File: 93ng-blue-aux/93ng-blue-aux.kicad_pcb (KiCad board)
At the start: 2 copper layers, 100 x 100 mm, 32 parts, among them J1 12V INPUT, J2 ESP32 UART, J3 ESP32 JTAG, J4 AUX OUT, J5 MIC IN, J6 BM62 UART, J7 I-BUS, SW1 SYS CONFIG, U1 ESP32-WROOM-32D, U2 BA33DD0T, U3 MC33897, U4 BM62SPKS1MC2-0001AA

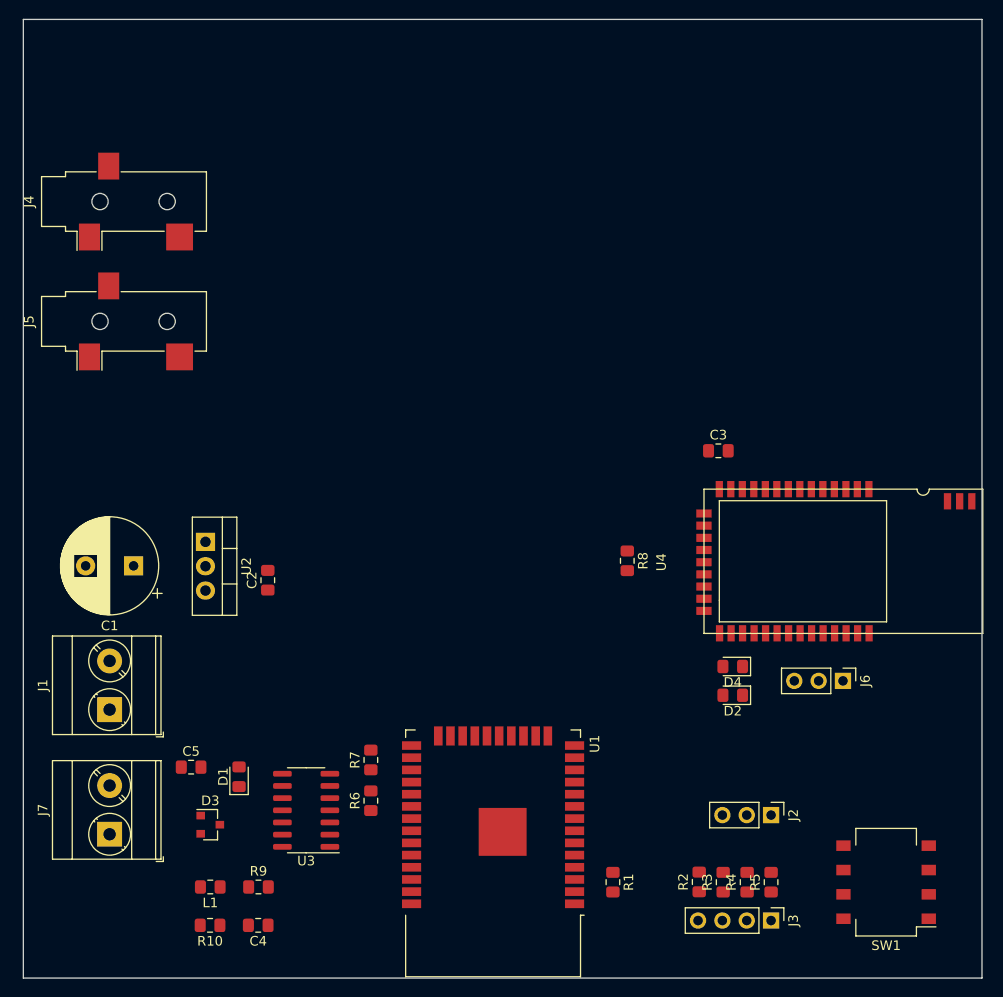
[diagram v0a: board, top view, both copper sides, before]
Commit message: PCB Layout progress.
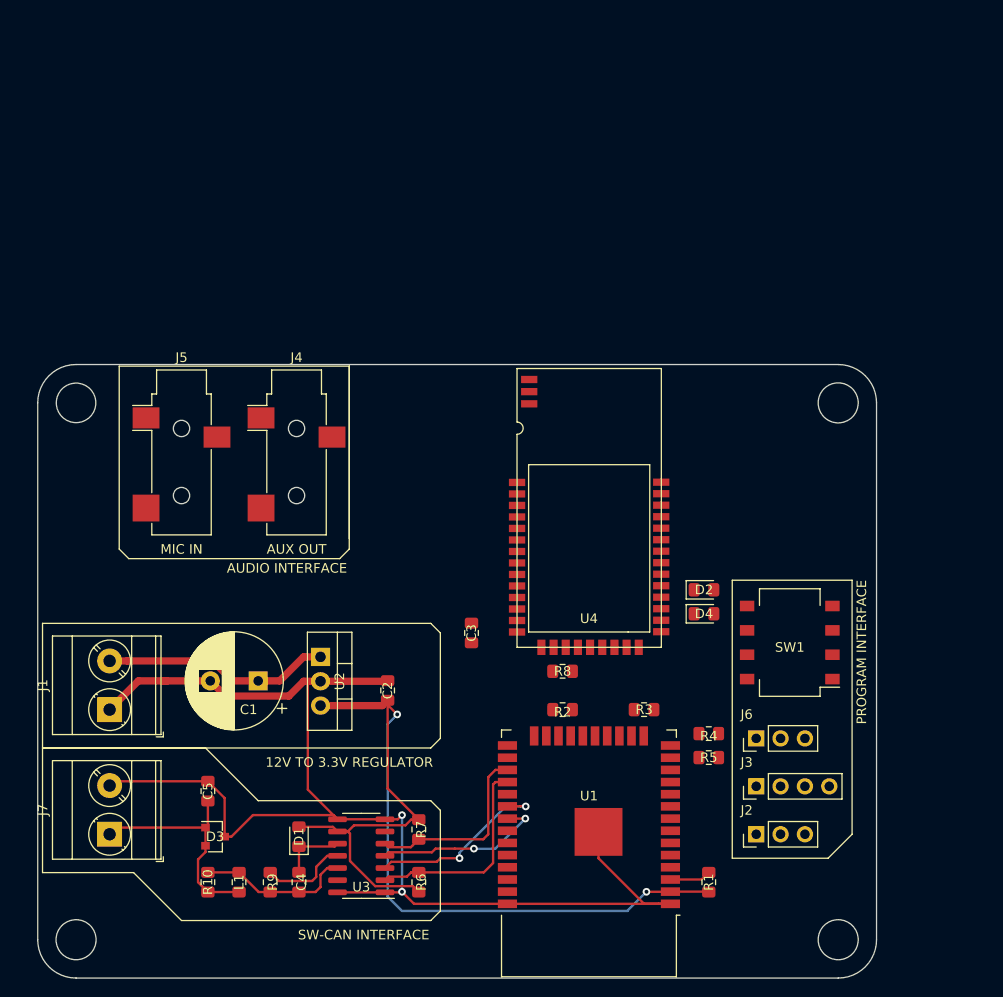
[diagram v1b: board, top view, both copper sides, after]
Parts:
- moved C3 32.0 mm to (95.8, 111.0), turned to 90 degrees
- moved J4 31.8 mm to (77.5, 92.2), turned to 0 degrees
- moved SW1 26.9 mm to (128.9, 112.0)
- moved U4 25.5 mm to (100.5, 112.5), turned to 0 degrees
- moved R2 22.9 mm to (105.2, 119.0), turned to 180 degrees
- moved R3 19.8 mm to (113.8, 119.0), turned to 180 degrees
- moved C1 17.7 mm to (73.5, 116.0)
- moved C2 17.0 mm to (87.0, 117.0)
- moved U2 17.0 mm to (80.0, 113.5)
- moved R4 16.0 mm to (120.5, 121.5), turned to 180 degrees
- moved J5 14.9 mm to (65.5, 92.2), turned to 0 degrees
- moved R5 14.5 mm to (120.5, 124.0), turned to 180 degrees
- moved J3 14.1 mm to (125.5, 127.0), turned to 90 degrees
- moved R8 13.4 mm to (105.2, 115.0), turned to 0 degrees
- moved D2 11.4 mm to (120.0, 106.5), turned to 0 degrees
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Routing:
- net GND: track 0.00 -> 141.2 mm, vias 0 -> 2
- net 3.3V: track 0.00 -> 102.2 mm, vias 0 -> 2
- net Net-(C1-Pad1): track 0.00 -> 23.9 mm
- net SW_CAN: track 0.00 -> 23.9 mm
- net MC33_TX: track 0.00 -> 21.8 mm
- net MC33_RX: track 0.00 -> 19.8 mm
- net MC33_MODE0: track 0.00 -> 19.6 mm, vias 0 -> 2
- net MC33_MODE1: track 0.00 -> 18.1 mm, vias 0 -> 2
- net Net-(C4-Pad2): track 0.00 -> 16.2 mm
- net Net-(R9-Pad2): track 0.00 -> 9.10 mm
- net Net-(C4-Pad1): track 0.00 -> 6.85 mm
- net Net-(R1-Pad1): track 0.00 -> 4.31 mm
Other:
- board size 100 x 100 mm -> 87.5 x 64 mm
- board text added: "12V TO 3.3V REGULATOR"
- board text added: "AUDIO INTERFACE"
- board text added: "PROGRAM INTERFACE"
- board text added: "SW-CAN INTERFACE"
